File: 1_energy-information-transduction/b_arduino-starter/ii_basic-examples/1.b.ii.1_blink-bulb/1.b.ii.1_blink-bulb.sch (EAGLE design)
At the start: 3 parts, among them T1 2N706

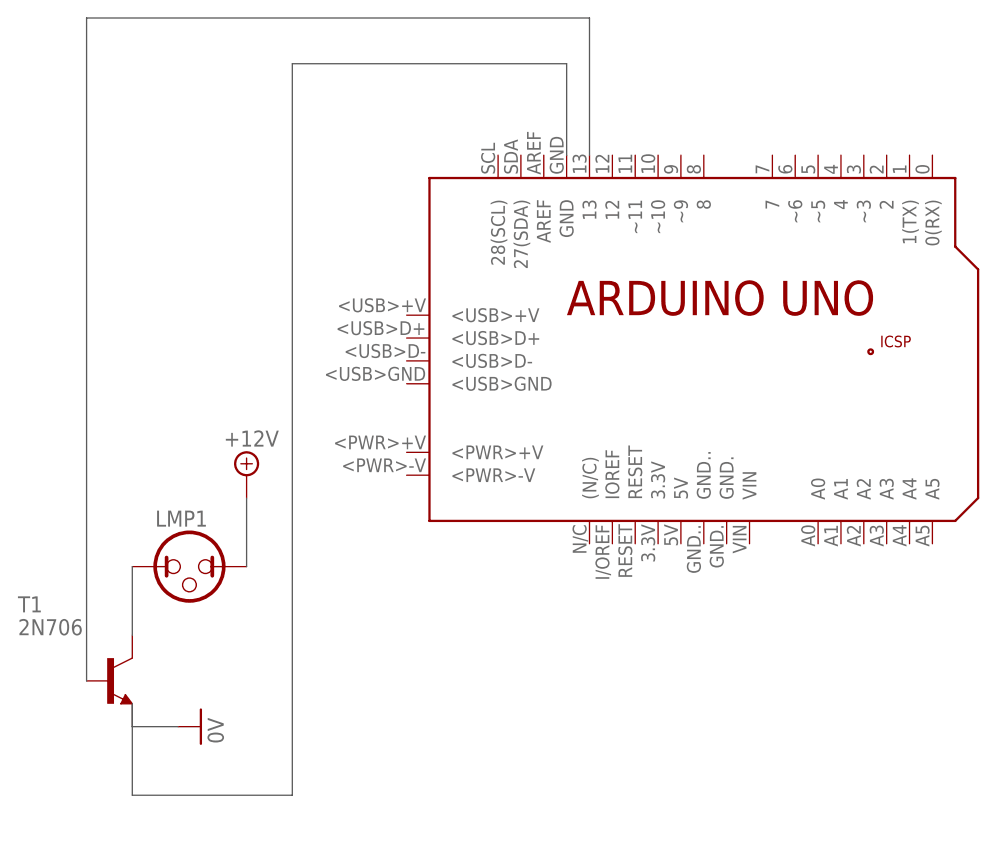
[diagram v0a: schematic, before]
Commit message: Bus to net.
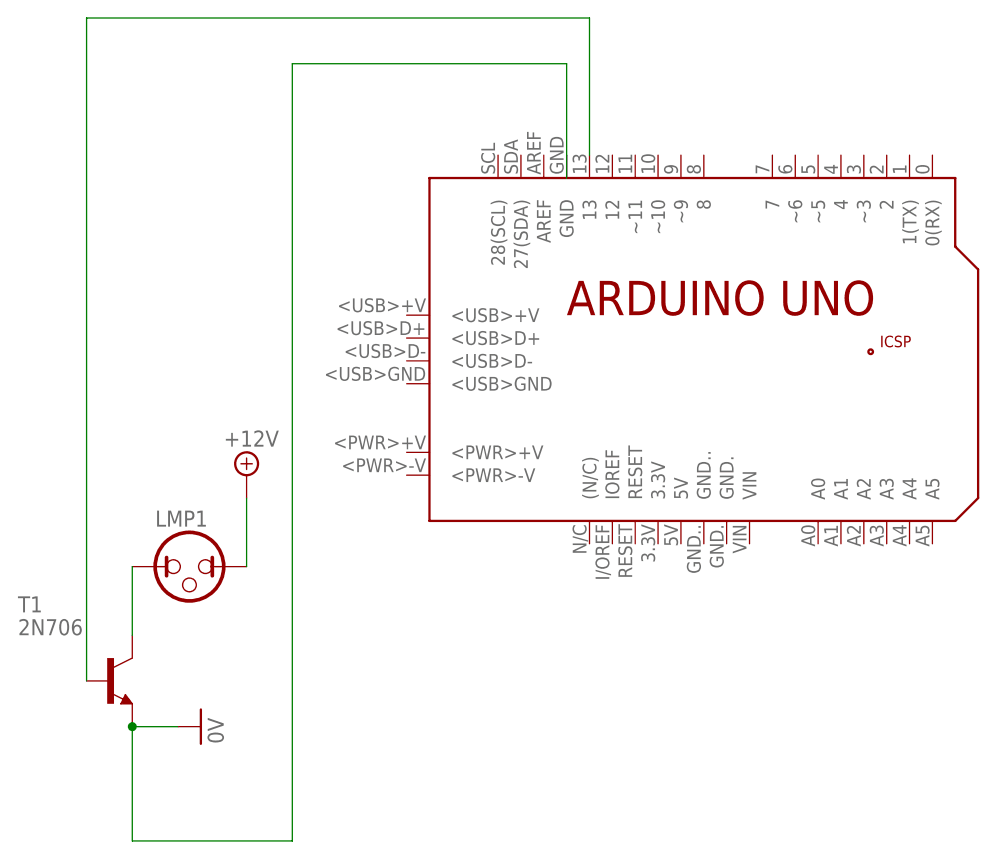
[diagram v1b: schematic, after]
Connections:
- new net +12V: LMP1.2
- new net 0V: T1.E
- new net N$1: LMP1.1, T1.C
- new net N$2: PCB1.13, T1.B
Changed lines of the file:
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@@
 </instances>
 <busses>
-<bus name="B$2">
-<segment>
-<wire x1="93.98" y1="50.8" x2="93.98" y2="66.04" width="0.762" layer="92"/>
-<wire x1="93.98" y1="66.04" x2="38.1" y2="66.04" width="0.762" layer="92"/>
-<wire x1="38.1" y1="66.04" x2="38.1" y2="-7.62" width="0.762" layer="92"/>
-</segment>
-</bus>
-<bus name="B$3">
-<segment>
-<wire x1="91.44" y1="50.8" x2="91.44" y2="60.96" width="0.762" layer="92"/>
-<wire x1="91.44" y1="60.96" x2="60.96" y2="60.96" width="0.762" layer="92"/>
-<wire x1="60.96" y1="60.96" x2="60.96" y2="-20.32" width="0.762" layer="92"/>
-<wire x1="60.96" y1="-20.32" x2="43.18" y2="-20.32" width="0.762" layer="92"/>
-<wire x1="43.18" y1="-20.32" x2="43.18" y2="-12.7" width="0.762" layer="92"/>
-<wire x1="48.26" y1="-12.7" x2="43.18" y2="-12.7" width="0.762" layer="92"/>
-<wire x1="43.18" y1="-12.7" x2="43.18" y2="-10.16" width="0.762" layer="92"/>
-</segment>
-</bus>
-<bus name="B$4">
-<segment>
-<wire x1="55.88" y1="12.7" x2="55.88" y2="5.08" width="0.762" layer="92"/>
-</segment>
-</bus>
-<bus name="B$5">
-<segment>
-<wire x1="43.18" y1="5.08" x2="43.18" y2="-2.54" width="0.762" layer="92"/>
-</segment>
-</bus>
 </busses>
 <nets>
+<net name="+12V" class="0">
+<segment>
+<pinref part="LMP1" gate="G$1" pin="2"/>
+<pinref part="SUPPLY1" gate="+12V" pin="+12V"/>
+<wire x1="55.88" y1="5.08" x2="55.88" y2="12.7" width="0.1524" layer="91"/>
+</segment>
+</net>
+<net name="N$1" class="0">
+<segment>
+<pinref part="T1" gate="G$1" pin="C"/>
+<pinref part="LMP1" gate="G$1" pin="1"/>
+<wire x1="43.18" y1="-2.54" x2="43.18" y2="5.08" width="0.1524" layer="91"/>
+</segment>
+</net>
+<net name="0V" class="0">
+<segment>
+<pinref part="T1" gate="G$1" pin="E"/>
+<pinref part="GND1" gate="1" pin="0V"/>
+<wire x1="43.18" y1="-12.7" x2="48.26" y2="-12.7" width="0.1524" layer="91"/>
+<wire x1="43.18" y1="-12.7" x2="43.18" y2="-25.4" width="0.1524" layer="91"/>
+<junction x="43.18" y="-12.7"/>
+<wire x1="43.18" y1="-25.4" x2="60.96" y2="-25.4" width="0.1524" layer="91"/>
+<wire x1="60.96" y1="-25.4" x2="60.96" y2="60.96" width="0.1524" layer="91"/>
+<wire x1="91.44" y1="50.8" x2="91.44" y2="48.26" width="0.1524" layer="91"/>
+<wire x1="60.96" y1="60.96" x2="91.44" y2="60.96" width="0.1524" layer="91"/>
+<wire x1="91.44" y1="60.96" x2="91.44" y2="50.8" width="0.1524" layer="91"/>
+</segment>
+</net>
+<net name="N$2" class="0">
+<segment>
+<pinref part="T1" gate="G$1" pin="B"/>
+<wire x1="38.1" y1="-7.62" x2="38.1" y2="66.04" width="0.1524" layer="91"/>
+<pinref part="PCB1" gate="G$1" pin="13"/>
+<wire x1="38.1" y1="66.04" x2="93.98" y2="66.04" width="0.1524" layer="91"/>
+<wire x1="93.98" y1="66.04" x2="93.98" y2="50.8" width="0.1524" layer="91"/>
+</segment>
+</net>
 </nets>
 </sheet>
